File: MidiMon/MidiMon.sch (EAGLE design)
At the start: 53 parts, among them IC1 PIC18F4520-I/P, IC2 6N138, IC5 7805TV, J1 DIN5, J2 DIN5, J4 2.1MMJACKTHM, X1 ECS-100-18-4X

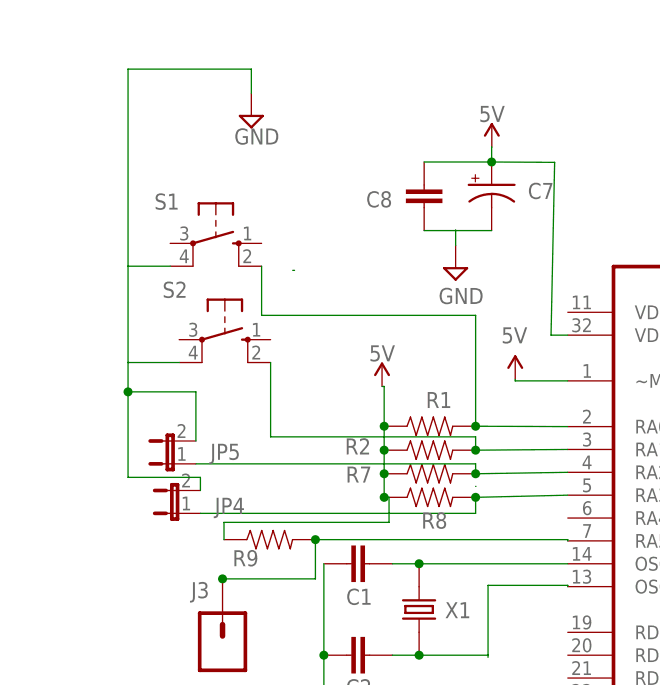
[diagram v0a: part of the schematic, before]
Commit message: More adjustments Signed-off-by: goslo <digit99@mailinator.com>
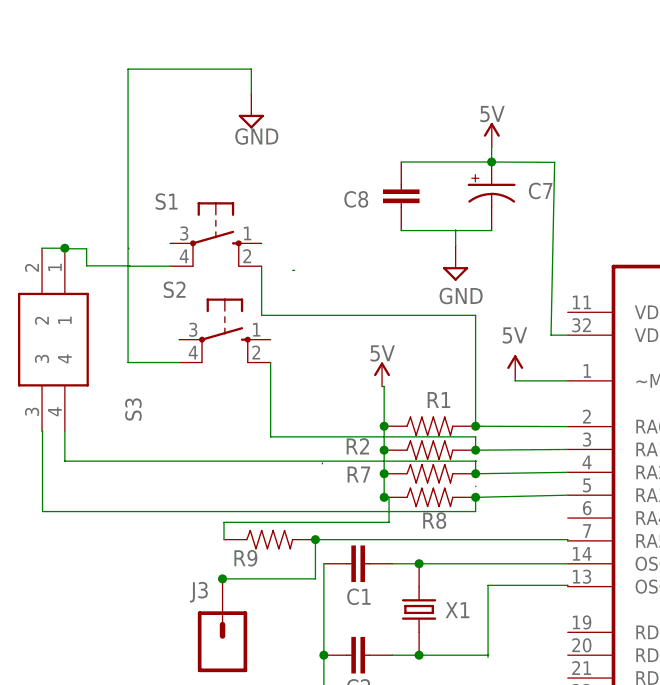
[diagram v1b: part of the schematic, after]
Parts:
- removed JP4, JP5: (no value), SparkFun-Retired:JUMPER-2PTH
- added S3: 195-2MST, SamacSys_Parts:195-2MST
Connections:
- removed net N$11: C7.-, C8.1
- removed net N$16: IC1.RA2/AN2/VREF-/CVREF, JP5.1, R7.2
- new net N$13: IC1.RA2/AN2/VREF-/CVREF, R7.2, S3.4
- net GND: now also C7.-, C8.1, S3.1, S3.2; no longer JP4.2, JP5.2
- net N$17: now also S3.3; no longer JP4.1
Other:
- moved on the sheet: C8
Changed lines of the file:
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@@
 <part name="SUPPLY6" library="supply2" library_urn="urn:adsk.eagle:library:372" deviceset="GND" device=""/>
 <part name="SUPPLY7" library="supply2" library_urn="urn:adsk.eagle:library:372" deviceset="GND" device=""/>
-<part name="JP4" library="SparkFun-Retired" deviceset="JUMPER-2" device="PTH"/>
-<part name="JP5" library="SparkFun-Retired" deviceset="JUMPER-2" device="PTH"/>
 <part name="SUPPLY8" library="supply2" library_urn="urn:adsk.eagle:library:372" deviceset="GND" device=""/>
 <part name="SUPPLY9" library="SparkFun-PowerSymbols" deviceset="5V" device=""/>
@@
 <part name="H4" library="SparkFun-Hardware" deviceset="STAND-OFF" device="TIGHT"/>
 <part name="J8" library="SparkFun-Connectors" library_urn="urn:adsk.eagle:library:513" deviceset="CONN_03" device="" package3d_urn="urn:adsk.eagle:package:38063/1"/>
+<part name="S3" library="SamacSys_Parts" deviceset="195-2MST" device=""/>
 </parts>
 <sheets>
@@
 <attribute name="NAME" x="18.416" y="129.935" size="1.778" layer="95" font="vector"/>
 </instance>
-<instance part="C8" gate="G$1" x="6.9" y="131.5" smashed="yes" rot="R180">
-<attribute name="NAME" x="3.376" y="130.779" size="1.778" layer="95" font="vector" rot="R180"/>
+<instance part="C8" gate="G$1" x="4.36" y="131.5" smashed="yes" rot="R180">
+<attribute name="NAME" x="0.836" y="130.779" size="1.778" layer="95" font="vector" rot="R180"/>
 </instance>
 <instance part="R6" gate="G$1" x="34.66" y="39.08" smashed="yes" rot="R90">
@@
 <instance part="SUPPLY7" gate="GND" x="15.7" y="53.84" smashed="yes">
 <attribute name="VALUE" x="13.795" y="50.665" size="1.778" layer="96"/>
-</instance>
-<instance part="JP4" gate="A" x="-20.5" y="95" smashed="yes" rot="R90">
-<attribute name="NAME" x="-13" y="96.73" size="1.778" layer="95" rot="R180"/>
-<attribute name="VALUE" x="-20.5" y="100.715" size="1.778" layer="96" rot="R180"/>
-</instance>
-<instance part="JP5" gate="A" x="-21" y="100.5" smashed="yes" rot="R90">
-<attribute name="NAME" x="-13.5" y="102.73" size="1.778" layer="95" rot="R180"/>
-<attribute name="VALUE" x="-21" y="106.215" size="1.778" layer="96" rot="R180"/>
 </instance>
 <instance part="SUPPLY8" gate="GND" x="-12.3" y="139.16" smashed="yes">
@@
 <attribute name="VALUE" x="170.434" y="177.8" size="1.778" layer="96" font="vector" rot="R270"/>
 <attribute name="NAME" x="170.18" y="173.228" size="1.778" layer="95" font="vector"/>
+</instance>
+<instance part="S3" gate="G$1" x="-33.02" y="124.46" smashed="yes" rot="R270">
+<attribute name="NAME" x="-25.4" y="107.95" size="1.778" layer="95" rot="R270" align="center-left"/>
 </instance>
 </instances>
@@
 <pinref part="S1" gate="1" pin="P1"/>
 <wire x1="-21.32" y1="122.46" x2="-26" y2="122.46" width="0.1524" layer="91"/>
-<pinref part="JP4" gate="A" pin="2"/>
-<wire x1="-17.96" y1="97.54" x2="-17.96" y2="99" width="0.1524" layer="91"/>
-<wire x1="-17.96" y1="99" x2="-26" y2="99" width="0.1524" layer="91"/>
-<wire x1="-26" y1="99" x2="-26" y2="108.5" width="0.1524" layer="91"/>
-<pinref part="JP5" gate="A" pin="2"/>
-<wire x1="-26" y1="108.5" x2="-26" y2="111.76" width="0.1524" layer="91"/>
-<wire x1="-18.46" y1="103.04" x2="-18.46" y2="108.5" width="0.1524" layer="91"/>
-<wire x1="-18.46" y1="108.5" x2="-26" y2="108.5" width="0.1524" layer="91"/>
-<junction x="-26" y="108.5"/>
 </segment>
 <segment>
@@
 <wire x1="192.46" y1="51.74" x2="192.46" y2="51.08" width="0.1524" layer="91"/>
 </segment>
+<segment>
+<pinref part="S3" gate="G$1" pin="2"/>
+<pinref part="S3" gate="G$1" pin="1"/>
+<wire x1="-35.56" y1="124.46" x2="-33.02" y2="124.46" width="0.1524" layer="91"/>
+<wire x1="-25.8" y1="122.5" x2="-30.6" y2="122.5" width="0.1524" layer="91"/>
+<wire x1="-30.6" y1="122.5" x2="-30.6" y2="124.4" width="0.1524" layer="91"/>
+<wire x1="-30.6" y1="124.4" x2="-33.02" y2="124.4" width="0.1524" layer="91"/>
+<wire x1="-33.02" y1="124.4" x2="-33.02" y2="124.46" width="0.1524" layer="91"/>
+<junction x="-33.02" y="124.46"/>
+</segment>
+<segment>
+<pinref part="C7" gate="G$1" pin="-"/>
+<pinref part="C8" gate="G$1" pin="1"/>
+<wire x1="14.4" y1="126.42" x2="4.36" y2="126.42" width="0.1524" layer="91"/>
+</segment>
 </net>
 <net name="N$4" class="0">
@@
 <pinref part="C8" gate="G$1" pin="2"/>
 <pinref part="C7" gate="G$1" pin="+"/>
-<wire x1="14.4" y1="134.04" x2="6.9" y2="134.04" width="0.1524" layer="91"/>
+<wire x1="14.4" y1="134.04" x2="4.36" y2="134.04" width="0.1524" layer="91"/>
 <wire x1="14.4" y1="134.04" x2="21.4" y2="134" width="0.1524" layer="91"/>
 <junction x="14.4" y="134.04"/>
@@
 </segment>
 </net>
-<net name="N$11" class="0">
-<segment>
-<pinref part="C7" gate="G$1" pin="-"/>
-<pinref part="C8" gate="G$1" pin="1"/>
-<wire x1="14.4" y1="126.42" x2="6.9" y2="126.42" width="0.1524" layer="91"/>
-</segment>
-</net>
 <net name="N$16" class="0">
 <segment>
-<pinref part="IC1" gate="A" pin="RA2/AN2/VREF-/CVREF"/>
-<pinref part="R7" gate="G$1" pin="2"/>
-<wire x1="22.86" y1="99.56" x2="12.62" y2="99.4" width="0.1524" layer="91"/>
-<wire x1="12.66" y1="99.4" x2="12.62" y2="99.4" width="0.1524" layer="91"/>
-<junction x="12.62" y="99.4"/>
-<pinref part="JP5" gate="A" pin="1"/>
-<wire x1="-18.46" y1="100.5" x2="12.62" y2="100.5" width="0.1524" layer="91"/>
-<wire x1="12.62" y1="100.5" x2="12.62" y2="99.4" width="0.1524" layer="91"/>
+<wire x1="-4.4" y1="100.5" x2="-4.4" y2="100.6" width="0.1524" layer="91"/>
 </segment>
 </net>
@@
 <wire x1="12.62" y1="96.78" x2="12.62" y2="96.5" width="0.1524" layer="91"/>
 <junction x="12.62" y="96.78"/>
-<pinref part="JP4" gate="A" pin="1"/>
-<wire x1="12.62" y1="96.78" x2="12.62" y2="95" width="0.1524" layer="91"/>
-<wire x1="12.62" y1="95" x2="-17.96" y2="95" width="0.1524" layer="91"/>
+<wire x1="12.62" y1="96.78" x2="12.62" y2="95.2" width="0.1524" layer="91"/>
+<wire x1="12.62" y1="95.2" x2="-35.5" y2="95.2" width="0.1524" layer="91"/>
+<pinref part="S3" gate="G$1" pin="3"/>
+<wire x1="-35.5" y1="95.2" x2="-35.5" y2="104.14" width="0.1524" layer="91"/>
+<wire x1="-35.5" y1="104.14" x2="-35.56" y2="104.14" width="0.1524" layer="91"/>
 </segment>
 </net>
@@
 </segment>
 </net>
+<net name="N$13" class="0">
+<segment>
+<pinref part="R7" gate="G$1" pin="2"/>
+<pinref part="IC1" gate="A" pin="RA2/AN2/VREF-/CVREF"/>
+<wire x1="22.86" y1="99.56" x2="12.62" y2="99.4" width="0.1524" layer="91"/>
+<wire x1="12.66" y1="99.4" x2="12.62" y2="99.4" width="0.1524" layer="91"/>
+<junction x="12.62" y="99.4"/>
+<wire x1="12.62" y1="99.4" x2="12.62" y2="100.8" width="0.1524" layer="91"/>
+<wire x1="12.62" y1="100.8" x2="12.7" y2="100.8" width="0.1524" layer="91"/>
+<pinref part="S3" gate="G$1" pin="4"/>
+<wire x1="12.62" y1="100.8" x2="-33.02" y2="100.8" width="0.1524" layer="91"/>
+<wire x1="-33.02" y1="100.8" x2="-33.02" y2="104.14" width="0.1524" layer="91"/>
+</segment>
+</net>
+<net name="N$32" class="0">
+<segment>
+<wire x1="-25.9" y1="124.46" x2="-25.9" y2="124.4" width="0.1524" layer="91"/>
+</segment>
+</net>
